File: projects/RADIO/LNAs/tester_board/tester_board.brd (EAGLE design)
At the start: 20 x 30 mm, 6 parts, among them X1 SMA-142-0711-821/826

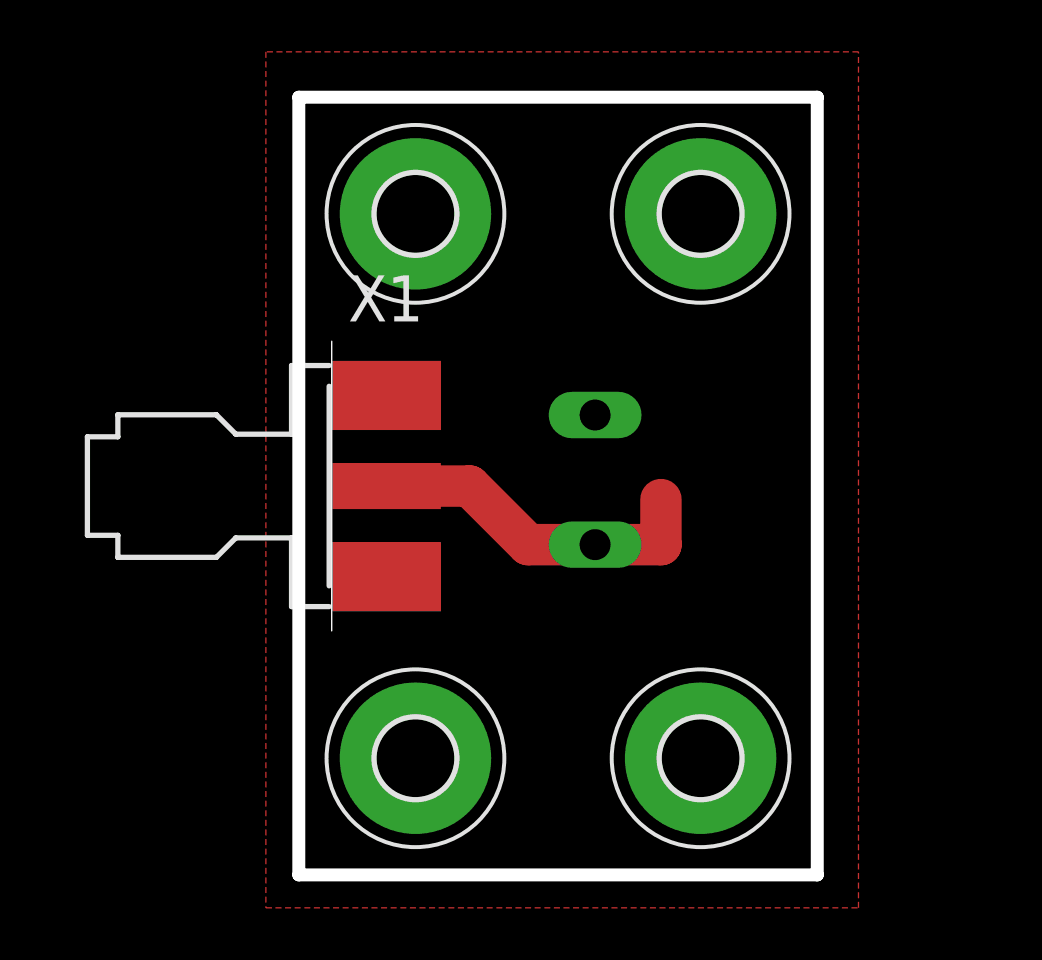
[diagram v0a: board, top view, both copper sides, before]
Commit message: update
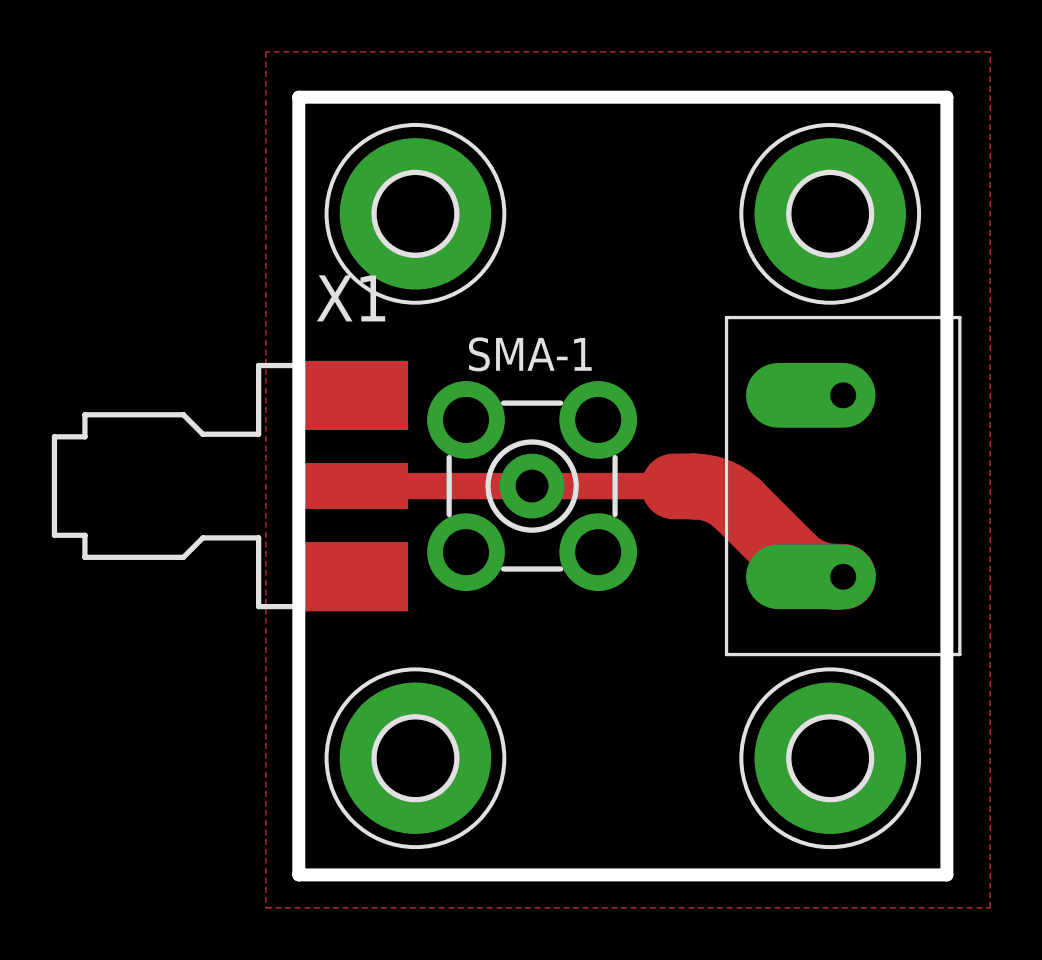
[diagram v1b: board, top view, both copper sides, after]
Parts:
- removed X2: (no value), con-wago-500:W237-102
- added CON1: CON_SCREW_CLAMP_7MM, mylib:CON_SCREW_CLAMP_7MM
- added SMA-1: SMA_TH, mylib:BU-SMA-V
- moved H3 5.00 mm to (20.5, 25.5)
- moved H4 5.00 mm to (20.5, 4.50)
- moved X1 1.27 mm to (0.00, 15.0)
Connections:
- net GND: now also CON1.P$2, SMA-1.2, SMA-1.3, SMA-1.4, SMA-1.5; no longer X2.1
- net N$1: now also CON1.P$1, SMA-1.1; no longer X2.2
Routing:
- net N$1: track 13.3 -> 20.0 mm
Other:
- board size 20 x 30 mm -> 25 x 30 mm
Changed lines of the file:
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@@
 <layer number="45" name="Holes" color="7" fill="1" visible="no" active="yes"/>
 <layer number="46" name="Milling" color="3" fill="1" visible="no" active="yes"/>
-<layer number="47" name="Measures" color="7" fill="1" visible="no" active="yes"/>
+<layer number="47" name="Measures" color="7" fill="1" visible="yes" active="yes"/>
 <layer number="48" name="Document" color="7" fill="1" visible="yes" active="yes"/>
 <layer number="49" name="Reference" color="7" fill="1" visible="yes" active="yes"/>
@@
 <board>
 <plain>
-<wire x1="0" y1="0" x2="20" y2="0" width="0.5" layer="20" locked="yes"/>
-<wire x1="20" y1="0" x2="20" y2="30" width="0.5" layer="20" locked="yes"/>
-<wire x1="20" y1="30" x2="0" y2="30" width="0.5" layer="20" locked="yes"/>
+<wire x1="0" y1="0" x2="25" y2="0" width="0.5" layer="20" locked="yes"/>
+<wire x1="25" y1="0" x2="25" y2="30" width="0.5" layer="20" locked="yes"/>
+<wire x1="25" y1="30" x2="0" y2="30" width="0.5" layer="20" locked="yes"/>
 <wire x1="0" y1="30" x2="0" y2="0" width="0.5" layer="20" locked="yes"/>
+<dimension x1="0" y1="30" x2="0" y2="0" x3="-12.7" y3="15" textsize="1.778" layer="47"/>
+<dimension x1="25" y1="30" x2="0" y2="30" x3="12.5" y3="34.29" textsize="1.778" layer="47"/>
 </plain>
 <attributes>
@@
 </autorouter>
 <elements>
-<element name="X1" library="con-coax" library_urn="urn:adsk.eagle:library:133" package="J502-ND-142-0711-821/826" package3d_urn="urn:adsk.eagle:package:6224/1" value="SMA-142-0711-821/826" x="1.27" y="15" smashed="yes">
-<attribute name="MF" value="JOHNSON COMPONENTS" x="43.18" y="4.84" size="1.778" layer="27" display="off"/>
-<attribute name="MPN" value="142-0711-821" x="43.18" y="4.84" size="1.778" layer="27" display="off"/>
-<attribute name="NAME" x="1.905" y="21.35" size="1.778" layer="25"/>
-<attribute name="OC_FARNELL" value="1019328" x="43.18" y="4.84" size="1.778" layer="27" display="off"/>
-<attribute name="OC_NEWARK" value="16F3627" x="43.18" y="4.84" size="1.778" layer="27" display="off"/>
-<attribute name="POPULARITY" value="0" x="43.18" y="4.84" size="1.778" layer="27" display="off"/>
-</element>
-<element name="X2" library="con-wago-500" library_urn="urn:adsk.eagle:library:195" package="W237-102" package3d_urn="urn:adsk.eagle:package:10688/1" value="" x="10.16" y="15.24" smashed="yes" rot="MR270">
-<attribute name="MF" value="" x="35.56" y="-2.54" size="1.778" layer="28" rot="MR270" display="off"/>
-<attribute name="MPN" value="237-102" x="35.56" y="-2.54" size="1.778" layer="28" rot="MR270" display="off"/>
-<attribute name="NAME" x="15.1638" y="19.0862" size="1.27" layer="26" ratio="10" rot="MR270"/>
-<attribute name="OC_FARNELL" value="unknown" x="35.56" y="-2.54" size="1.778" layer="28" rot="MR270" display="off"/>
-<attribute name="OC_NEWARK" value="70K9898" x="35.56" y="-2.54" size="1.778" layer="28" rot="MR270" display="off"/>
-<attribute name="POPULARITY" value="32" x="35.56" y="-2.54" size="1.778" layer="28" rot="MR270" display="off"/>
-<attribute name="VALUE" x="17.78" y="20.28" size="1.27" layer="28" ratio="10" rot="MR270"/>
+<element name="X1" library="con-coax" library_urn="urn:adsk.eagle:library:133" package="J502-ND-142-0711-821/826" package3d_urn="urn:adsk.eagle:package:6224/1" value="SMA-142-0711-821/826" x="0" y="15" smashed="yes">
+<attribute name="MF" value="JOHNSON COMPONENTS" x="41.91" y="4.84" size="1.778" layer="27" display="off"/>
+<attribute name="MPN" value="142-0711-821" x="41.91" y="4.84" size="1.778" layer="27" display="off"/>
+<attribute name="NAME" x="0.635" y="21.35" size="1.778" layer="25"/>
+<attribute name="OC_FARNELL" value="1019328" x="41.91" y="4.84" size="1.778" layer="27" display="off"/>
+<attribute name="OC_NEWARK" value="16F3627" x="41.91" y="4.84" size="1.778" layer="27" display="off"/>
+<attribute name="POPULARITY" value="0" x="41.91" y="4.84" size="1.778" layer="27" display="off"/>
 </element>
 <element name="H1" library="holes" library_urn="urn:adsk.eagle:library:237" package="3,0-PAD" package3d_urn="urn:adsk.eagle:package:14280/1" value="MOUNT-PAD-ROUND3.0" x="4.5" y="4.5" locked="yes" smashed="yes">
@@
 <attribute name="POPULARITY" value="17" x="4.5" y="25.5" locked="yes" size="1.778" layer="27" display="off"/>
 </element>
-<element name="H3" library="holes" library_urn="urn:adsk.eagle:library:237" package="3,0-PAD" package3d_urn="urn:adsk.eagle:package:14280/1" value="MOUNT-PAD-ROUND3.0" x="15.5" y="25.5" locked="yes" smashed="yes">
-<attribute name="POPULARITY" value="17" x="15.5" y="25.5" locked="yes" size="1.778" layer="27" display="off"/>
-</element>
-<element name="H4" library="holes" library_urn="urn:adsk.eagle:library:237" package="3,0-PAD" package3d_urn="urn:adsk.eagle:package:14280/1" value="MOUNT-PAD-ROUND3.0" x="15.5" y="4.5" locked="yes" smashed="yes">
-<attribute name="POPULARITY" value="17" x="15.5" y="4.5" locked="yes" size="1.778" layer="27" display="off"/>
+<element name="H3" library="holes" library_urn="urn:adsk.eagle:library:237" package="3,0-PAD" package3d_urn="urn:adsk.eagle:package:14280/1" value="MOUNT-PAD-ROUND3.0" x="20.5" y="25.5" locked="yes" smashed="yes">
+<attribute name="POPULARITY" value="17" x="20.5" y="25.5" locked="yes" size="1.778" layer="27" display="off"/>
+</element>
+<element name="H4" library="holes" library_urn="urn:adsk.eagle:library:237" package="3,0-PAD" package3d_urn="urn:adsk.eagle:package:14280/1" value="MOUNT-PAD-ROUND3.0" x="20.5" y="4.5" locked="yes" smashed="yes">
+<attribute name="POPULARITY" value="17" x="20.5" y="4.5" locked="yes" size="1.778" layer="27" display="off"/>
+</element>
+<element name="CON1" library="mylib" package="CON_SCREW_CLAMP_7MM" value="CON_SCREW_CLAMP_7MM" x="21" y="15" smashed="yes" rot="R90"/>
+<element name="SMA-1" library="mylib" package="BU-SMA-V" value="SMA_TH" x="9" y="15" smashed="yes">
+<attribute name="NAME" x="6.46" y="19.445" size="1.27" layer="25"/>
+<attribute name="VALUE" x="5.825" y="9.285" size="1.27" layer="27"/>
 </element>
 </elements>
@@
 <signal name="N$1">
 <contactref element="X1" pad="1"/>
-<contactref element="X2" pad="2"/>
-<wire x1="3.3854" y1="15" x2="6.59" y2="15" width="1.6" layer="1"/>
-<wire x1="11.43" y1="12.74" x2="8.85" y2="12.74" width="1.6" layer="1"/>
-<wire x1="8.85" y1="12.74" x2="6.59" y2="15" width="1.6" layer="1"/>
-<wire x1="11.43" y1="12.74" x2="13.97" y2="12.74" width="1.6" layer="1"/>
-<wire x1="13.97" y1="12.74" x2="13.97" y2="14.478" width="1.6" layer="1"/>
+<contactref element="CON1" pad="P$1"/>
+<contactref element="SMA-1" pad="1"/>
+<wire x1="2.1154" y1="15" x2="9" y2="15" width="1.016" layer="1"/>
+<wire x1="9" y1="15" x2="14.478" y2="15" width="1.016" layer="1"/>
+<wire x1="14.478" y1="15" x2="14.478" y2="14.986" width="1.016" layer="1"/>
+<wire x1="14.478" y1="14.986" x2="15.24" y2="14.986" width="2.54" layer="1"/>
+<wire x1="15.24" y1="14.986" x2="16.974425" y2="14.267575" width="2.54" layer="1" curve="-45"/>
+<wire x1="19.044275" y1="12.197725" x2="20.72873125" y2="11.5" width="2.54" layer="1" curve="45"/>
+<wire x1="20.72873125" y1="11.5" x2="21" y2="11.5" width="2.54" layer="1"/>
+<wire x1="16.974425" y1="14.267575" x2="19.044275" y2="12.197725" width="2.54" layer="1"/>
 </signal>
 <signal name="GND">
@@
 <contactref element="X1" pad="G@3"/>
 <contactref element="X1" pad="G@4"/>
-<contactref element="X2" pad="1"/>
-<polygon width="0.5" layer="1" isolate="1.5" locked="yes">
+<polygon width="0.5" layer="1" pour="hatch" isolate="1.5" locked="yes">
 <vertex x="-1.27" y="31.75"/>
 <vertex x="-1.27" y="-1.27"/>
-<vertex x="21.59" y="-1.27"/>
-<vertex x="21.59" y="31.75"/>
+<vertex x="26.67" y="-1.27"/>
+<vertex x="26.67" y="31.75"/>
 </polygon>
 <contactref element="H1" pad="B3,0"/>
@@
 <contactref element="H3" pad="B3,0"/>
 <contactref element="H4" pad="B3,0"/>
-<wire x1="3.3854" y1="18.4946" x2="3.3854" y2="18.4946" width="0" layer="19" extent="1-16"/>
-<wire x1="3.3854" y1="11.5054" x2="3.3854" y2="11.5054" width="0" layer="19" extent="1-16"/>
+<contactref element="CON1" pad="P$2"/>
+<contactref element="SMA-1" pad="3"/>
+<contactref element="SMA-1" pad="4"/>
+<contactref element="SMA-1" pad="2"/>
+<contactref element="SMA-1" pad="5"/>
+<wire x1="2.1154" y1="18.4946" x2="2.1154" y2="18.4946" width="0" layer="19" extent="1-16"/>
+<wire x1="6.4501" y1="12.4501" x2="6.4501" y2="17.5499" width="0" layer="19" extent="1-1"/>
+<wire x1="2.1154" y1="11.5054" x2="2.1154" y2="11.5054" width="0" layer="19" extent="1-16"/>
 </signal>
 </signals>
@@
 <mfgpreviewcolor name="substratecolor" color="0xFF786E46"/>
 </mfgpreviewcolors>
+<errors>
+</errors>
 </board>
 </drawing>
